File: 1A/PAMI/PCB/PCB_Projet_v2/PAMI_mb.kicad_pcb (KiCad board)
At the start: 4 copper layers, 65 x 56 mm, 107 parts, among them J1 Conn_02x20_Odd_Even, J10 Conn_01x04, J11 Conn_01x04, J12 Conn_01x04, J13 Conn_01x04, J2 Conn_01x03, J3 Conn_ST_STDC14, J4 Battery, J5 Charge, J6 Stop, J8 173010542, J9 Conn_01x04, SW1 SW_Push_SPDT, SW2 RotaryEncoder_Switch, SW3 SW_Push, SW4 SW_Push, SW5 SW_Push, SW6 SW_Push, U1 STM32G431KBTx, U2 LT1076CR-PBF, U3 AZ1117CH2-3.3TRG1, U4 TMC2225-SA-T, U5 TMC2225-SA-T

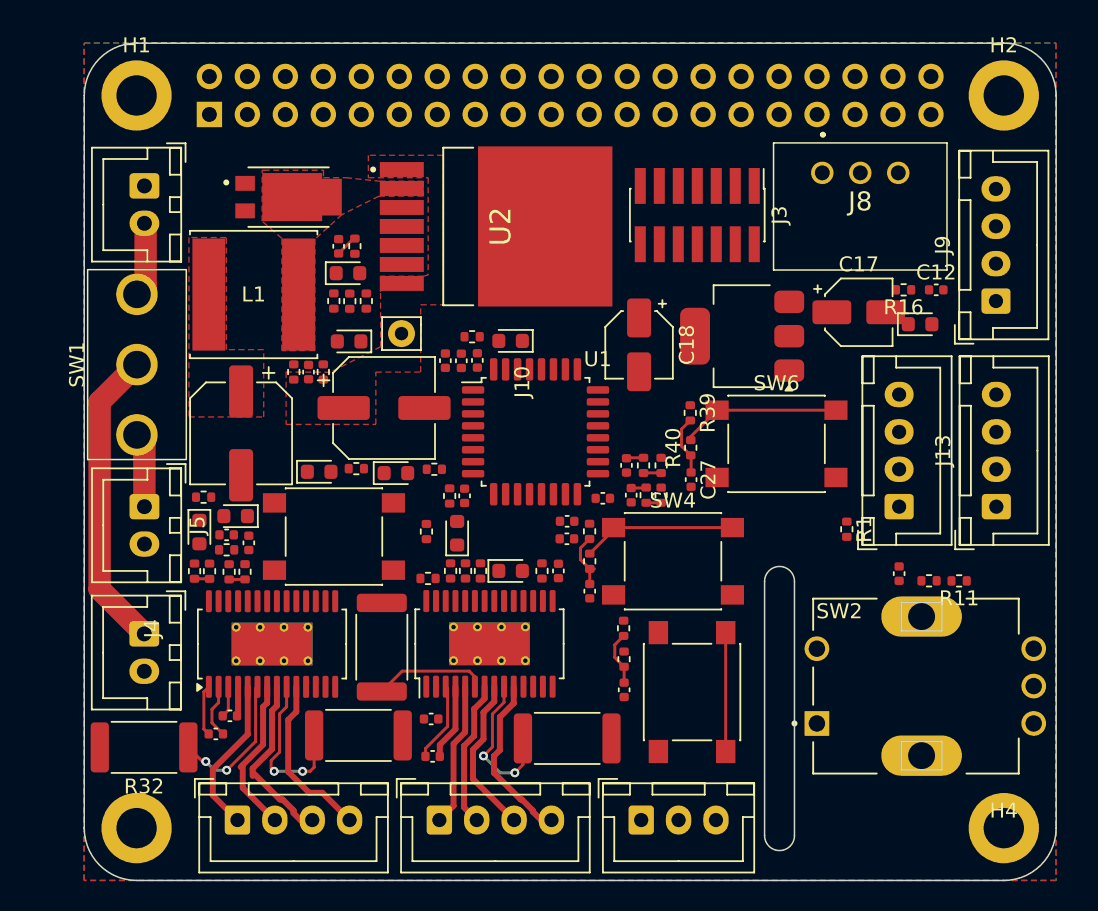
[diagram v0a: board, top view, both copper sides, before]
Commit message: update PAMI pcb
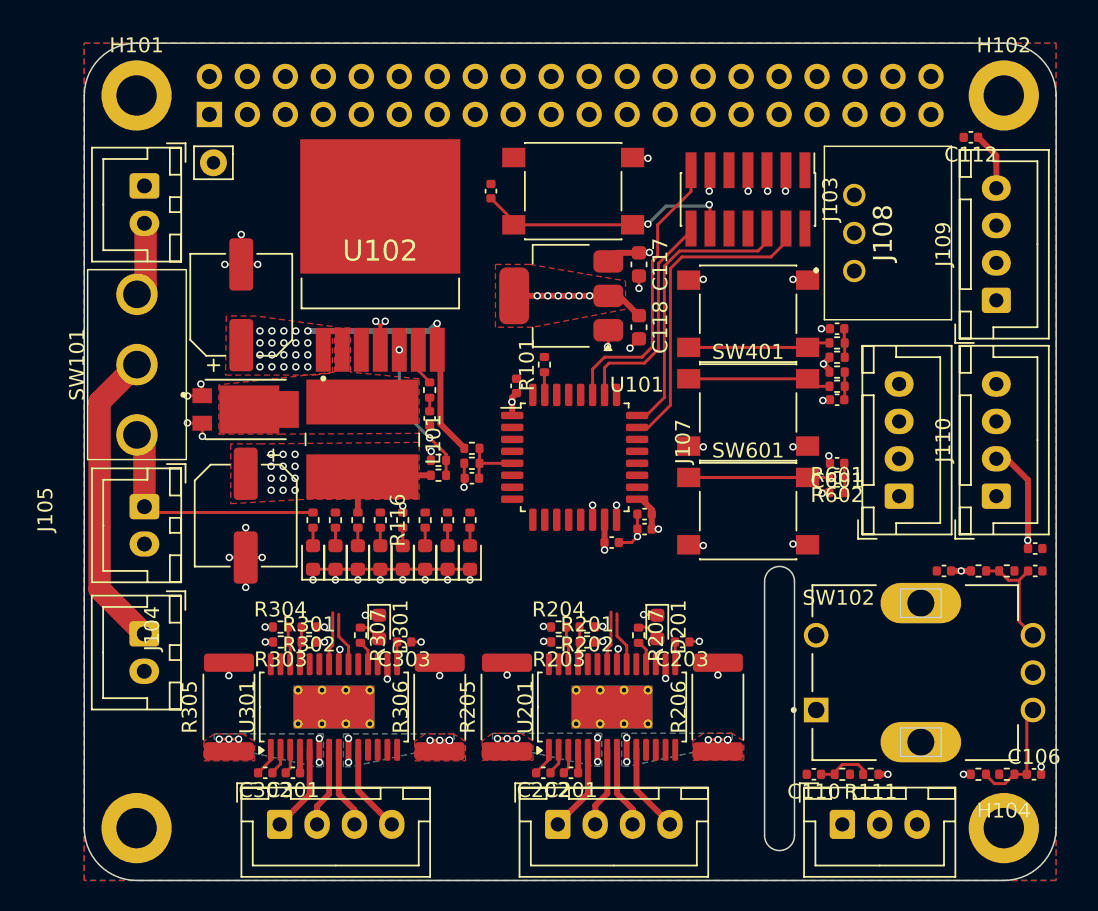
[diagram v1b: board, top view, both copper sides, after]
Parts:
- removed C10, C6: 10n, Capacitor_SMD:C_0402_1005Metric
- removed C17, C18: 10u, Capacitor_SMD:CP_Elec_4x5.4
- removed C19, C22: 100nF, Capacitor_SMD:C_0402_1005Metric
- removed C20, C23: 22nF, Capacitor_SMD:C_0402_1005Metric
- removed C21, C24: 2.2uF, Capacitor_SMD:C_0402_1005Metric
- removed C8: 10u, Capacitor_SMD:C_0402_1005Metric
- removed D10, D9: LED, LED_SMD:LED_0603_1608Metric
- removed J10: Conn_01x04, Connector_JST:JST_XH_B4B-XH-A_1x04_P2.50mm_Vertical
- removed R21, R22, R23, R24, R28, R29, R30, R31: 0R, Resistor_SMD:R_0402_1005Metric
- removed R25, R26, R32, R33: 150m, Resistor_SMD:R_2512_6332Metric
- removed R27, R34: 1k, Resistor_SMD:R_0402_1005Metric
- removed U4, U5: TMC2225-SA-T, Package_SO:HTSSOP-28-1EP_4.4x9.7mm_P0.65mm_EP2.85x5.4mm_ThermalVias
- added C106: 10n, Capacitor_SMD:C_0402_1005Metric, F.Cu at (190.0, 95.4)
- added C110: 10n, Capacitor_SMD:C_0402_1005Metric, F.Cu at (175.3, 95.4)
- added C117: 10u, Capacitor_SMD:C_0603_1608Metric, F.Cu at (163.6, 61.3)
- added C118: 10u, Capacitor_SMD:C_0603_1608Metric, F.Cu at (163.6, 65.5)
- added C201: 100nF, Capacitor_SMD:C_0402_1005Metric, F.Cu at (159.1, 95.3)
- added C202: 22nF, Capacitor_SMD:C_0402_1005Metric, F.Cu at (157.2, 95.3)
- added C203: 2.2uF, Capacitor_SMD:C_0402_1005Metric, F.Cu at (166.5, 86.5)
- added C301: 100nF, Capacitor_SMD:C_0402_1005Metric, F.Cu at (140.5, 95.3)
- added C302: 22nF, Capacitor_SMD:C_0402_1005Metric, F.Cu at (138.6, 95.3)
- added C303: 2.2uF, Capacitor_SMD:C_0402_1005Metric, F.Cu at (147.9, 86.5)
- added D201: LED, LED_SMD:LED_0603_1608Metric, F.Cu at (164.8, 85.5)
- added D301: LED, LED_SMD:LED_0603_1608Metric, F.Cu at (146.2, 85.5)
- added J110: Conn_01x04, Connector_JST:JST_XH_B4B-XH-A_1x04_P2.50mm_Vertical, F.Cu at (187.5, 76.8)
- added R201: 0R, Resistor_SMD:R_0402_1005Metric, F.Cu at (160.1, 86.5)
- added R202: 0R, Resistor_SMD:R_0402_1005Metric, F.Cu at (160.1, 85.5)
- added R203: 0R, Resistor_SMD:R_0402_1005Metric, F.Cu at (158.2, 86.5)
- added R204: 0R, Resistor_SMD:R_0402_1005Metric, F.Cu at (158.2, 85.5)
- added R205: 150m, Resistor_SMD:R_2512_6332Metric, F.Cu at (154.8, 90.9)
- added R206: 150m, Resistor_SMD:R_2512_6332Metric, F.Cu at (168.9, 90.9)
- added R207: 1k, Resistor_SMD:R_0402_1005Metric, F.Cu at (163.6, 86.1)
- added R301: 0R, Resistor_SMD:R_0402_1005Metric, F.Cu at (141.5, 86.5)
- added R302: 0R, Resistor_SMD:R_0402_1005Metric, F.Cu at (141.5, 85.5)
- added R303: 0R, Resistor_SMD:R_0402_1005Metric, F.Cu at (139.6, 86.5)
- added R304: 0R, Resistor_SMD:R_0402_1005Metric, F.Cu at (139.6, 85.5)
- added R305: 150m, Resistor_SMD:R_2512_6332Metric, F.Cu at (136.2, 90.9)
- added R306: 150m, Resistor_SMD:R_2512_6332Metric, F.Cu at (150.3, 90.9)
- added R307: 1k, Resistor_SMD:R_0402_1005Metric, F.Cu at (145.0, 86.1)
- added U201: TMC2225-SA-T, Package_SO:HTSSOP-28-1EP_4.4x9.7mm_P0.65mm_EP2.85x5.4mm_ThermalVias, F.Cu at (161.8, 90.9)
- added U301: TMC2225-SA-T, Package_SO:HTSSOP-28-1EP_4.4x9.7mm_P0.65mm_EP2.85x5.4mm_ThermalVias, F.Cu at (143.2, 90.9)
- L101: renamed from L1; footprint Inductor_SMD:L_Changjiang_FNR8065S -> Inductor_SMD:L_Wuerth_WE-PD2-Typ-L
- moved C113 41.4 mm to (190.1, 80.3), turned to 0 degrees
- moved D106 39.3 mm to (146.3, 80.9), turned to 90 degrees
- moved R116 38.2 mm to (146.3, 78.4), turned to -90 degrees
- moved R105 30.5 mm to (188.2, 95.4), turned to 0 degrees
- moved C109 28.6 mm to (153.7, 56.4), turned to 90 degrees
- moved R109 28.3 mm to (186.3, 95.4), turned to 180 degrees
- moved C105 28.2 mm to (190.1, 81.8), turned to 0 degrees
- moved SW103 28.1 mm to (159.2, 56.4), turned to 180 degrees
- moved C501 28.0 mm to (176.8, 65.6), turned to 180 degrees
- moved SW501 25.6 mm to (170.9, 64.6), turned to 180 degrees
- moved R502 25.5 mm to (176.8, 66.5), turned to 180 degrees
- moved R103 25.3 mm to (188.2, 81.8), turned to 180 degrees
- moved C107 23.3 mm to (184.0, 81.8)
- moved R501 23.1 mm to (176.8, 67.5), turned to 0 degrees
- moved R101 23.0 mm to (157.3, 68.0), turned to 90 degrees
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- renumbered C1 to C101, C2 to C102, C3 to C103, C4 to C104, C5 to C105, C7 to C107, C9 to C109, C11 to C111, C12 to C112, C13 to C113, C14 to C114, C15 to C115, C16 to C116, C25 to C401, C26 to C501, C27 to C601, CR1 to CR101, D1 to D101, D2 to D102, D3 to D103, D4 to D104, D5 to D105, D6 to D106, D7 to D107, D8 to D108, H1 to H101, H2 to H102, H3 to H103, H4 to H104, J1 to J101, J2 to J102, J3 to J103, J4 to J104, J5 to J105, J6 to J106, J13 to J107, J8 to J108, J9 to J109, J11 to J111, J12 to J112, R1 to R101, R2 to R102, R5 to R103, R3 to R104, R4 to R105, R6 to R106, R7 to R107, R8 to R108, R9 to R109, R10 to R110, R11 to R111, R13 to R112, R14 to R113, R12 to R114, R15 to R115, R16 to R116, R17 to R117, R18 to R118, R19 to R119, R20 to R120, R35 to R401, R36 to R402, R37 to R501, R38 to R502, R39 to R601, R40 to R602, SW1 to SW101, SW2 to SW102, SW3 to SW103, SW4 to SW401, SW5 to SW501, SW6 to SW601, TP1 to TP101, U1 to U101, U2 to U102, U3 to U103
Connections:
- C105 pad 1: /ENCODEUR_B -> Net-(C105-Pad1)
- R103 pad 2: Net-(R5-Pad2) -> Net-(C105-Pad1)
- R107 pad 1: Net-(R5-Pad2) -> Net-(C105-Pad1)
- R111 pad 2: Net-(R11-Pad2) -> Net-(C110-Pad1)
- R114 pad 1: Net-(R11-Pad2) -> Net-(C110-Pad1)
- SW102 pad B: Net-(R5-Pad2) -> Net-(C105-Pad1)
- SW102 pad S1: Net-(R11-Pad2) -> GND
- SW102 pad S2: GND -> Net-(C110-Pad1)
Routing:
- net GND: track 0.00 -> 68.4 mm, vias 0 -> 57
- net VCC: track 7.13 -> 70.9 mm, vias 0 -> 21
- net +5V: track 0.00 -> 41.3 mm, vias 0 -> 1
- net +3.3V: track 0.00 -> 33.4 mm, vias 0 -> 23
- net /SWDIO: track 0.00 -> 21.4 mm
- net /SWCLK: track 0.00 -> 19.5 mm
- net /STLINK_RX: track 0.00 -> 19.2 mm
- net /NRST: track 0.00 -> 17.7 mm, vias 0 -> 2
- net /STLINK_TX: track 0.00 -> 14.9 mm
- net /V_CHARGE: track 5.01 -> 16.4 mm
- net Net-(U5-BRB): track 11.1 -> 0.00 mm, vias 2 -> 0
- net Net-(U4-BRB): track 10.3 -> 0.00 mm, vias 2 -> 0
- net /VFB: track 0.00 -> 9.69 mm, vias 0 -> 2
- net Net-(U5-BRA): track 9.63 -> 0.00 mm, vias 2 -> 0
- net Net-(U4-BRA): track 7.60 -> 0.00 mm
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- added copper zone on F.Cu, net +3.3V
- added copper zone on In1.Cu, net +3.3V
- added copper zone on In1.Cu, net +5.1V
- added copper zone on B.Cu, net Net-(U301-BRA)
- added copper zone on F.Cu, net Net-(U301-BRA)
- added copper zone on B.Cu, net Net-(U301-BRB)
- added copper zone on F.Cu, net Net-(U301-BRB)
- added copper zone on In1.Cu, net VCC
